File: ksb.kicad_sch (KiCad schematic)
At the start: 20 parts, among them J10 Conn_01x02, J11 Conn_02x08_Top_Bottom, J12 Conn_02x08_Top_Bottom, J4 Conn_02x08_Top_Bottom, J5 Conn_02x08_Top_Bottom, J7 Conn_02x08_Top_Bottom, J9 Conn_01x02

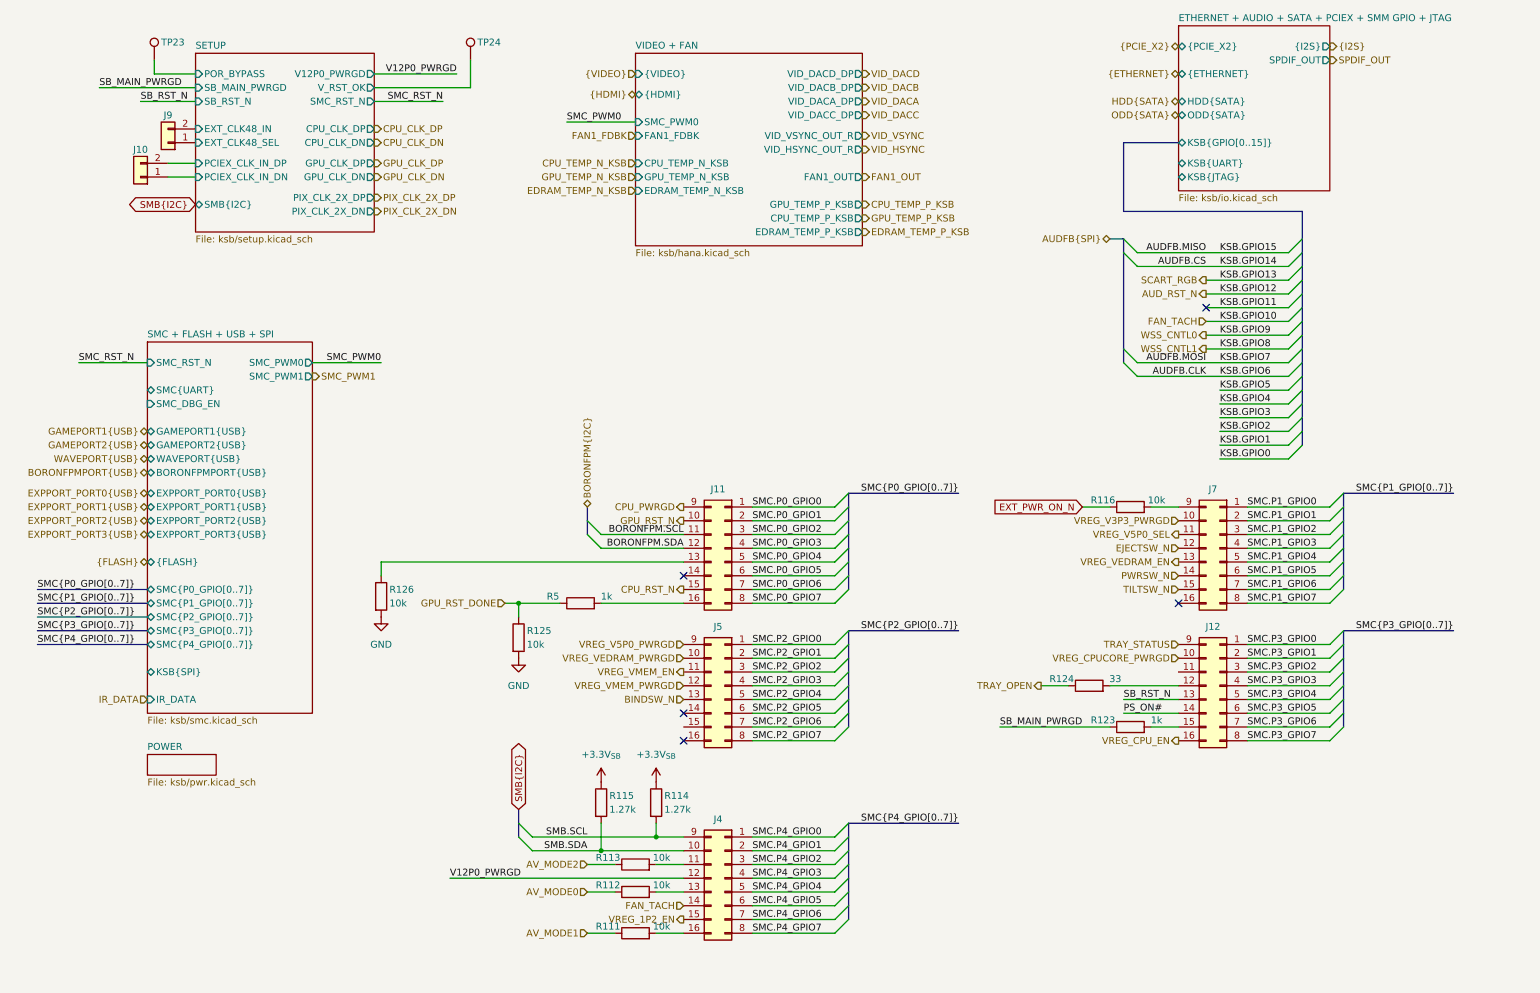
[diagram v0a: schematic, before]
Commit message: Cleanup & Debug I/O
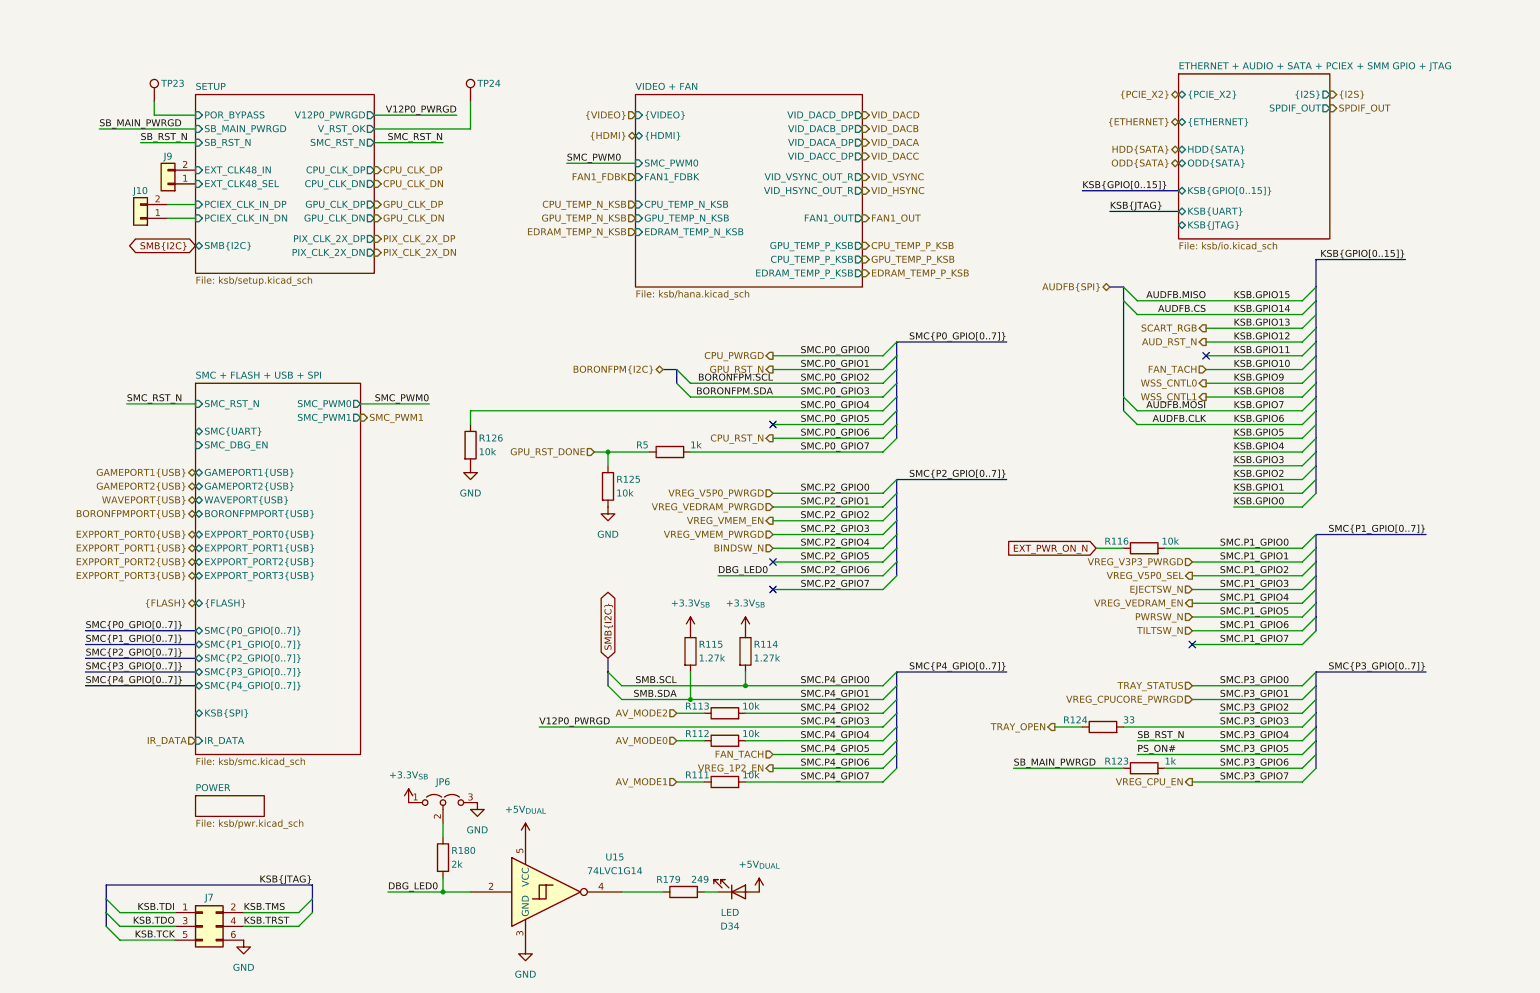
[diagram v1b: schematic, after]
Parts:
- removed J11, J12, J4, J5, J7: Conn_02x08_Top_Bottom, symbol Connector_Generic:Conn_02x08_Top_Bottom
- added D34: LED, symbol Device:LED
- added J7: Conn_02x03_Odd_Even, symbol Connector_Generic:Conn_02x03_Odd_Even
- added JP6: Jumper_3_Open, symbol Jumper:Jumper_3_Open
- added R179: 249, symbol Device:R
- added R180: 2k, symbol Device:R
- added U15: 74LVC1G14, symbol 74xGxx:74LVC1G14
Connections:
- net +3.3V_{SB}: now also JP6.1 (A)
- net GND: now also J7.6 (Pin_6), JP6.3 (B), U15.3 (GND)
- net SMC.P0_GPIO4: now also R126.1
- net SMC.P0_GPIO7: now also R5.2
- net SMC.P1_GPIO0: now also R116.2
- net SMC.P3_GPIO3: now also R124.2
- net SMC.P3_GPIO6: now also R123.2
- net SMC.P4_GPIO2: now also R113.2
- net SMC.P4_GPIO4: now also R112.2
- net SMC.P4_GPIO7: now also R111.2
- new net: JP6.2 (C), R180.1
- new net: R179.1, U15.4
- new net: D34.1 (K), R179.2
- new net +5V_{DUAL}: D34.2 (A), U15.5 (VCC)
- new net DBG_LED0: R180.2, U15.2
- new net KSB.TCK: J7.5 (Pin_5)
- new net KSB.TDI: J7.1 (Pin_1)
- new net KSB.TDO: J7.3 (Pin_3)
- new net KSB.TMS: J7.2 (Pin_2)
- new net KSB.TRST: J7.4 (Pin_4)
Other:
- moved on the sheet: J10, J9, R111, R112, R113, R114, R115, R116, R123, R124, R125, R126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
